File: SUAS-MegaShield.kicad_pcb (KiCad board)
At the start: 2 copper layers, 1 part

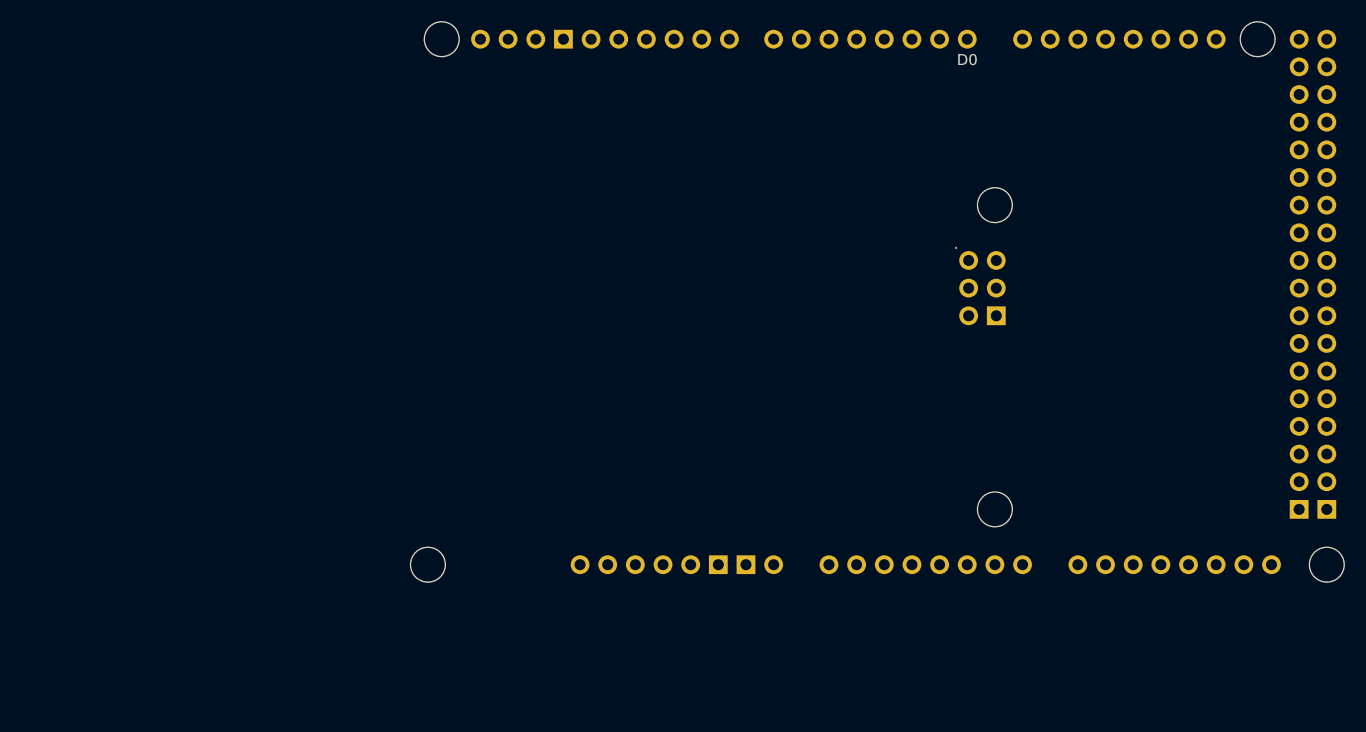
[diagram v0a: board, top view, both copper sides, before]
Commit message: autosave
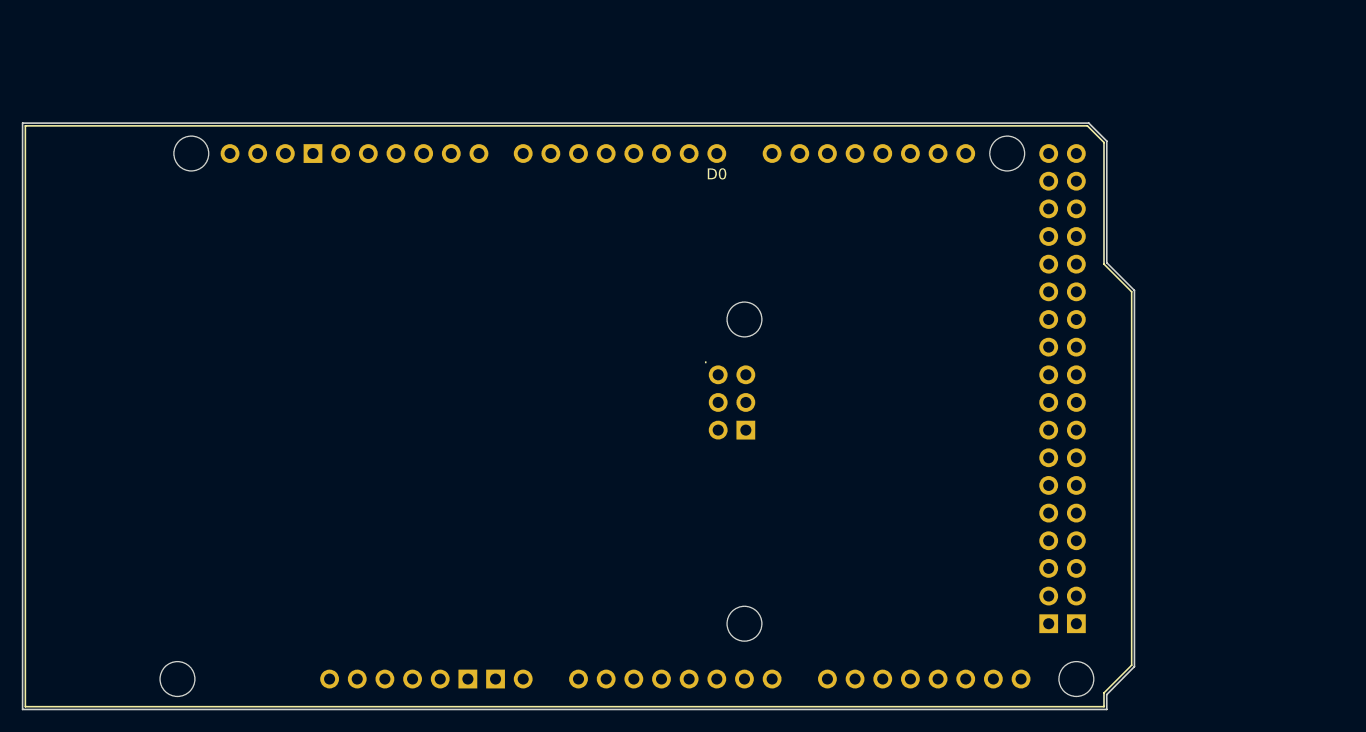
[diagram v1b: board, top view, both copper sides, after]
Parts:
- added ?: , clipboard:5463372f-7f41-4771-be05-13c3a7f8540b, F.Cu at (71.2, 82.4)
- A1: value Arduino_Giga_R1_WiFi_Shield -> Arduino_Mega_Shield
- moved A1 25.3 mm to (71.5, 136.0)
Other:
- board outline added: 102.1 x 53.8 mm
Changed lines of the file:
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@@
 	(footprint "arduino-library:Arduino_Giga_R1_WiFi_Shield"
 		(layer "F.Cu")
-		(at 94.48 125.54)
+		(at 71.48 136.04)
 		(descr "https://docs.arduino.cc/hardware/giga-r1-wifi")
 		(property "Reference" "A1"
@@
 			)
 		)
-		(property "Value" "Arduino_Giga_R1_WiFi_Shield"
+		(property "Value" "Arduino_Mega_Shield"
 			(at 27.305 -54.356 0)
 			(layer "B.Fab")
@@
 				(type solid)
 			)
-			(layer "B.SilkS")
+			(layer "F.SilkS")
 		)
 		(fp_line
@@
 				(type solid)
 			)
-			(layer "B.SilkS")
+			(layer "F.SilkS")
 		)
 		(fp_line
@@
 				(type solid)
 			)
-			(layer "B.SilkS")
+			(layer "F.SilkS")
 		)
 		(fp_line
@@
 				(type solid)
 			)
-			(layer "B.SilkS")
+			(layer "F.SilkS")
 		)
 		(fp_line
@@
 				(type solid)
 			)
-			(layer "B.SilkS")
+			(layer "F.SilkS")
 		)
 		(fp_line
@@
 				(type solid)
 			)
-			(layer "B.SilkS")
+			(layer "F.SilkS")
 		)
 		(fp_line
@@
 				(type solid)
 			)
-			(layer "B.SilkS")
+			(layer "F.SilkS")
 		)
 		(fp_line
@@
 				(type solid)
 			)
-			(layer "B.SilkS")
+			(layer "F.SilkS")
 		)
 		(fp_line
@@
 				(type solid)
 			)
-			(layer "B.SilkS")
+			(layer "F.SilkS")
 		)
 		(fp_line
@@
 			(fill none)
 			(layer "F.Fab")
-		)
-		(fp_text user "."
-			(at 62.484 -32.004 0)
-			(layer "B.SilkS")
-			(effects
-				(font
-					(size 1 1)
-					(thickness 0.15)
-				)
-			)
 		)
 		(fp_text user "D0"
@@
 		(fp_text user "."
 			(at 62.484 -32.004 0)
+			(layer "B.SilkS")
+			(effects
+				(font
+					(size 1 1)
+					(thickness 0.15)
+				)
+			)
+		)
+		(fp_text user "."
+			(at 62.484 -32.004 0)
 			(layer "F.SilkS")
 			(effects
@@
 			)
 		)
-		(fp_text user "Audio Jack"
-			(at 5 -9.515 0)
+		(fp_text user "USB C"
+			(at 2.665 -39.5 0)
 			(layer "B.Fab")
 			(effects
@@
 			)
 		)
-		(fp_text user "USB C"
-			(at 2.665 -39.5 0)
+		(fp_text user "Audio Jack"
+			(at 5 -9.515 0)
 			(layer "B.Fab")
 			(effects
@@
 		)
 	)
+	(footprint "clipboard:5463372f-7f41-4771-be05-13c3a7f8540b"
+		(layer "F.Cu")
+		(at 71.226 82.446)
+		(property "Reference" ""
+			(at 0 0 0)
+			(layer "F.SilkS")
+			(effects
+				(font
+					(size 1.27 1.27)
+					(thickness 0.15)
+				)
+			)
+		)
+		(property "Value" ""
+			(at 0 0 0)
+			(layer "F.Fab")
+			(effects
+				(font
+					(size 1.27 1.27)
+					(thickness 0.15)
+				)
+			)
+		)
+		(property "Footprint" ""
+			(at 0 0 0)
+			(layer "F.Fab")
+			(hide yes)
+			(effects
+				(font
+					(size 1.27 1.27)
+					(thickness 0.15)
+				)
+			)
+		)
+		(property "Datasheet" ""
+			(at 0 0 0)
+			(layer "F.Fab")
+			(hide yes)
+			(effects
+				(font
+					(size 1.27 1.27)
+					(thickness 0.15)
+				)
+			)
+		)
+		(property "Description" ""
+			(at 0 0 0)
+			(layer "F.Fab")
+			(hide yes)
+			(effects
+				(font
+					(size 1.27 1.27)
+					(thickness 0.15)
+				)
+			)
+		)
+		(fp_line
+			(start 0 53.848)
+			(end 0 0)
+			(stroke
+				(width 0.15)
+				(type solid)
+			)
+			(layer "Edge.Cuts")
+		)
+		(fp_line
+			(start 97.917 0)
+			(end 0 0)
+			(stroke
+				(width 0.15)
+				(type solid)
+			)
+			(layer "Edge.Cuts")
+		)
+		(fp_line
+			(start 99.564 52.484)
+			(end 99.568 53.848)
+			(stroke
+				(width 0.15)
+				(type solid)
+			)
+			(layer "Edge.Cuts")
+		)
+		(fp_line
+			(start 99.568 1.651)
+			(end 97.917 0)
+			(stroke
+				(width 0.15)
+				(type solid)
+			)
+			(layer "Edge.Cuts")
+		)
+		(fp_line
+			(start 99.568 1.651)
+			(end 99.568 12.827)
+			(stroke
+				(width 0.15)
+				(type solid)
+			)
+			(layer "Edge.Cuts")
+		)
+		(fp_line
+			(start 99.568 12.827)
+			(end 102.108 15.367)
+			(stroke
+				(width 0.15)
+				(type solid)
+			)
+			(layer "Edge.Cuts")
+		)
+		(fp_line
+			(start 99.568 53.848)
+			(end 0 53.848)
+			(stroke
+				(width 0.15)
+				(type solid)
+			)
+			(layer "Edge.Cuts")
+		)
+		(fp_line
+			(start 102.108 15.367)
+			(end 102.108 49.911)
+			(stroke
+				(width 0.15)
+				(type solid)
+			)
+			(layer "Edge.Cuts")
+		)
+		(fp_line
+			(start 102.108 49.911)
+			(end 99.564 52.484)
+			(stroke
+				(width 0.15)
+				(type solid)
+			)
+			(layer "Edge.Cuts")
+		)
+	)
